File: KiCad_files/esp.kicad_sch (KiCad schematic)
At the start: 18 parts, among them J2 USB_C_Receptacle_USB2.0_16P, Q1 DMP3099L, SW1 SW_Push, U1 ESP32-S3-MINI-1U, U2 BNO055, U6 LTC4412xS6

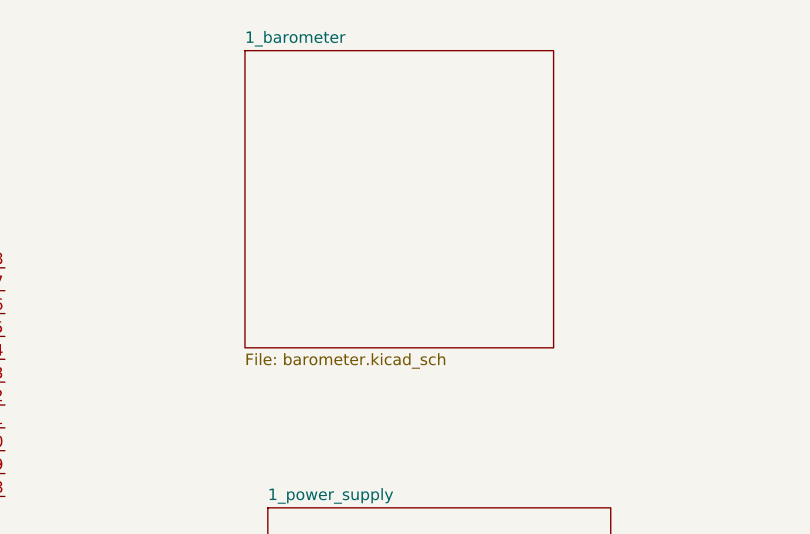
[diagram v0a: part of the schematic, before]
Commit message: barometri
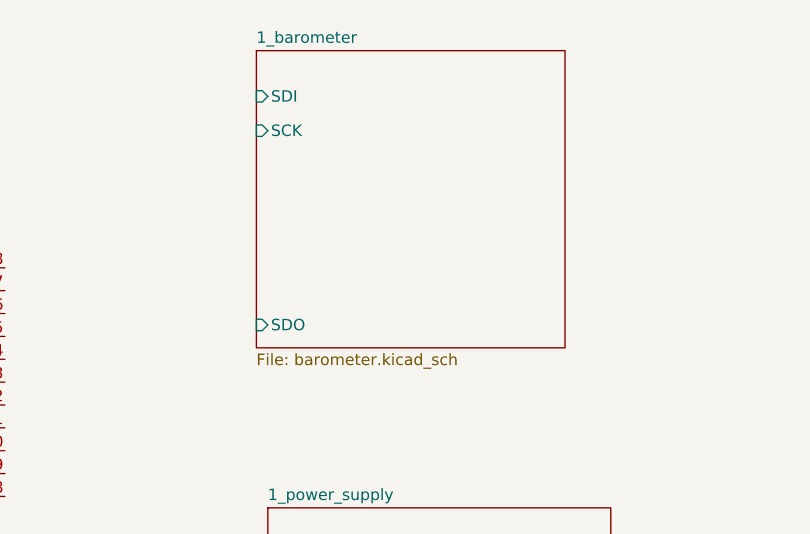
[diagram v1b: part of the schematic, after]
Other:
- sheet 1_barometer ports: added SCK, SDI, SDO; removed none
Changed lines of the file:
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@@
 	)
 	(sheet
-		(at 254 40.64)
+		(at 255.27 40.64)
 		(size 34.29 33.02)
 		(exclude_from_sim no)
@@
 		)
 		(property "Sheetname" "1_barometer"
-			(at 254 39.9284 0)
+			(at 255.27 39.9284 0)
 			(effects
 				(font
@@
 		)
 		(property "Sheetfile" "barometer.kicad_sch"
-			(at 254 74.2446 0)
+			(at 255.27 74.2446 0)
 			(effects
 				(font
@@
 			)
 		)
+		(pin "SCK" input
+			(at 255.27 49.53 180)
+			(effects
+				(font
+					(size 1.27 1.27)
+				)
+				(justify left)
+			)
+		)
+		(pin "SDI" input
+			(at 255.27 45.72 180)
+			(effects
+				(font
+					(size 1.27 1.27)
+				)
+				(justify left)
+			)
+		)
+		(pin "SDO" input
+			(at 255.27 71.12 180)
+			(effects
+				(font
+					(size 1.27 1.27)
+				)
+				(justify left)
+			)
+		)
